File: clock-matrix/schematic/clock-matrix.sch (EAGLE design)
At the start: 85 parts, among them IC1 WS2811-SOP8, IC2 WS2811-SOP8, IC3 74HC595D, U2 ATMEGA328P-MU, X2 USB-MICROB

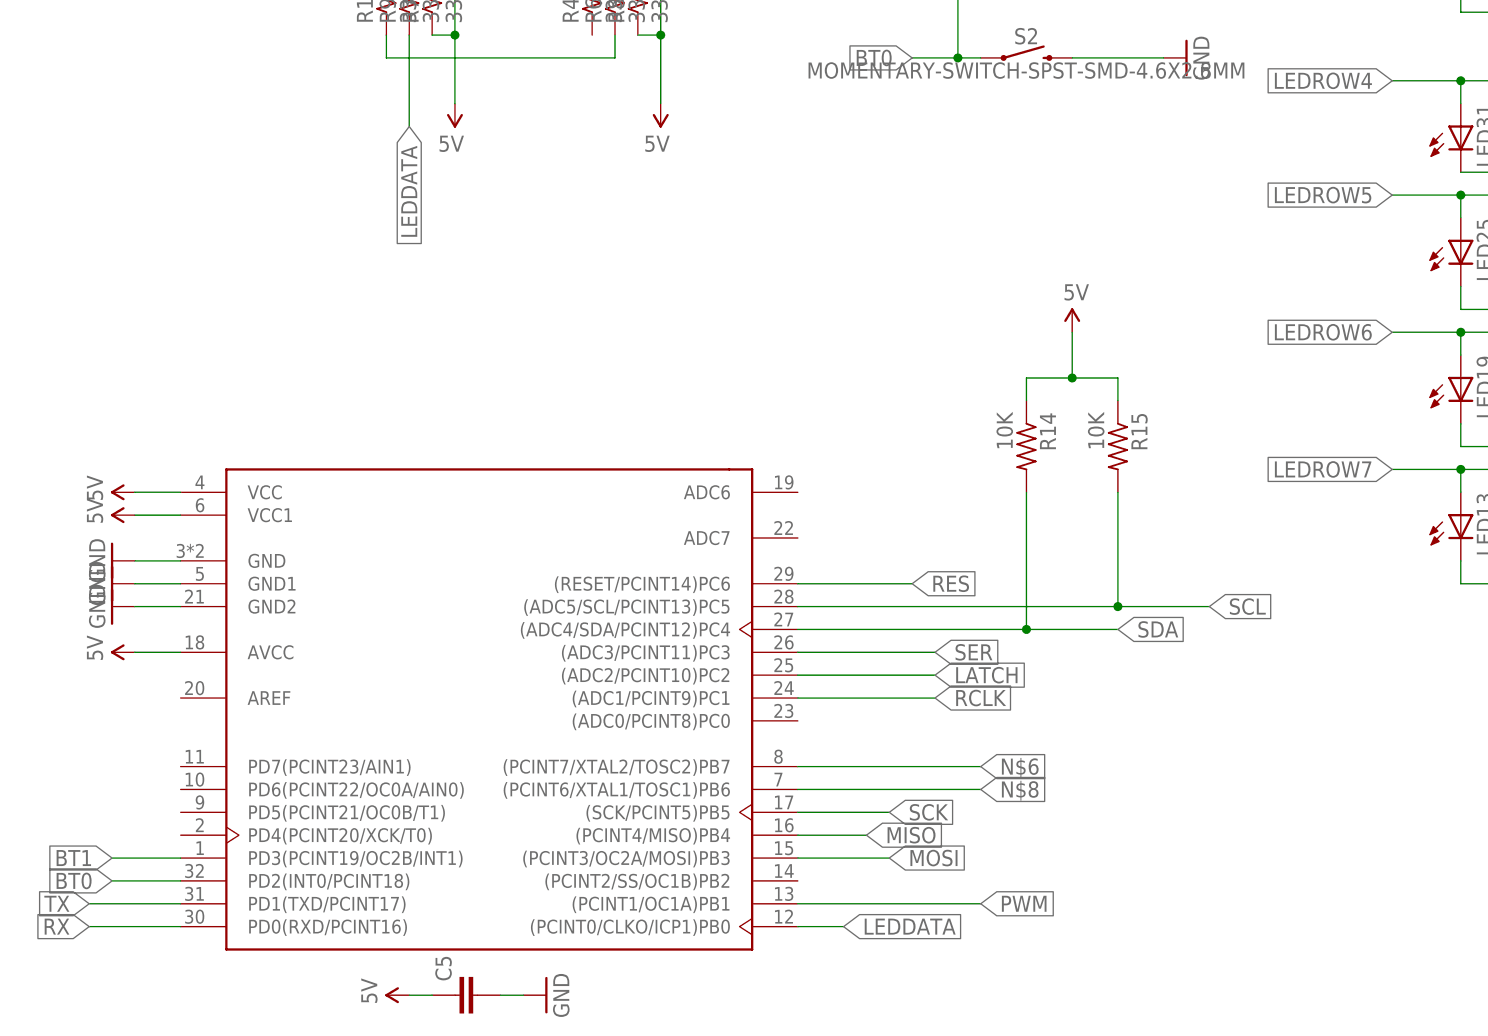
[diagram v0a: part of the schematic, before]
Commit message: Improvement, fixes and other changes
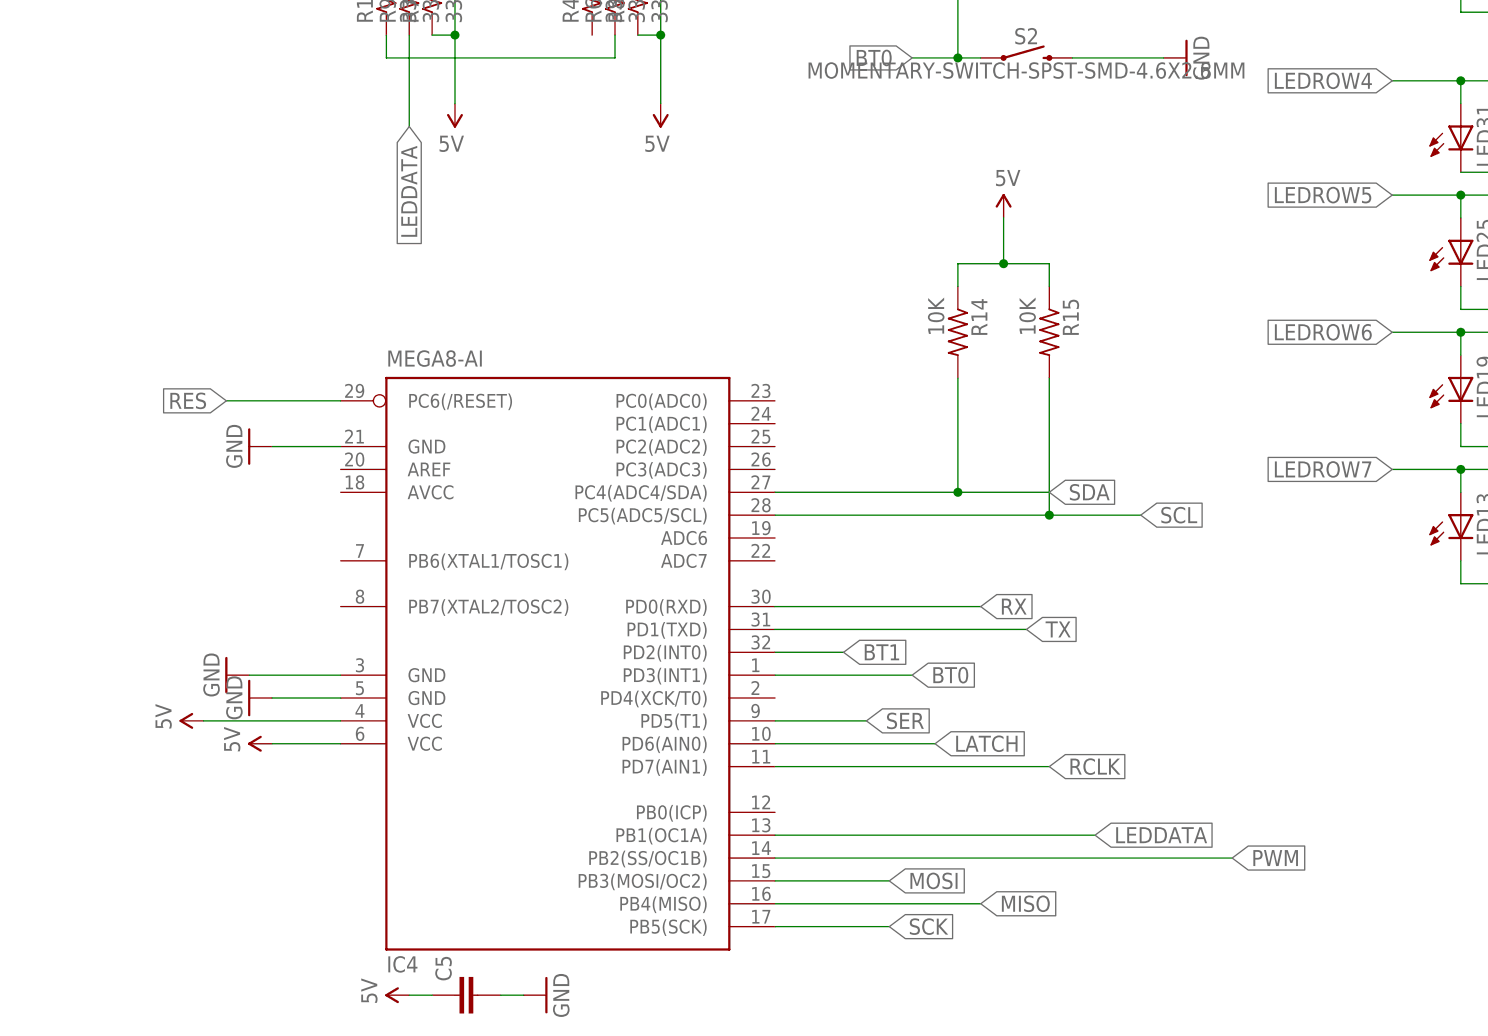
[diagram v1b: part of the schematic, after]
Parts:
- removed U2: ATMEGA328P-MU, Microcontroller:ATMEGA328P-MU
- added IC4: MEGA8-AI, atmel:MEGA8-AI
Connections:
- removed net N$6: U2.(PCINT7/XTAL2/TOSC2)PB7
- removed net N$8: U2.(PCINT6/XTAL1/TOSC1)PB6
- net 5V: now also IC4.VCC@1, IC4.VCC@2; no longer U2.AVCC, U2.VCC, U2.VCC1
- net BT0: now also IC4.PD3(INT1); no longer U2.PD2(INT0/PCINT18)
- net BT1: now also IC4.PD2(INT0); no longer U2.PD3(PCINT19/OC2B/INT1)
- net GND: now also IC4.GND, IC4.GND@1, IC4.GND@2; no longer U2.GND, U2.GND1, U2.GND2
- net LATCH: now also IC4.PD6(AIN0); no longer U2.(ADC2/PCINT10)PC2
- net LEDDATA: now also IC4.PB1(OC1A); no longer U2.(PCINT0/CLKO/ICP1)PB0
- net MISO: now also IC4.PB4(MISO); no longer U2.(PCINT4/MISO)PB4
- net MOSI: now also IC4.PB3(MOSI/OC2); no longer U2.(PCINT3/OC2A/MOSI)PB3
- net PWM: now also IC4.PB2(SS/OC1B); no longer U2.(PCINT1/OC1A)PB1
- net RCLK: now also IC4.PD7(AIN1); no longer U2.(ADC1/PCINT9)PC1
- net RES: now also IC4.PC6(/RESET); no longer U2.(RESET/PCINT14)PC6
- net RX: now also IC4.PD0(RXD); no longer U2.PD0(RXD/PCINT16)
- net SCK: now also IC4.PB5(SCK); no longer U2.(SCK/PCINT5)PB5
- net SCL: now also IC4.PC5(ADC5/SCL); no longer U2.(ADC5/SCL/PCINT13)PC5
- net SDA: now also IC4.PC4(ADC4/SDA); no longer U2.(ADC4/SDA/PCINT12)PC4
- net SER: now also IC4.PD5(T1); no longer U2.(ADC3/PCINT11)PC3
- net TX: now also IC4.PD1(TXD); no longer U2.PD1(TXD/PCINT17)
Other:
- moved on the sheet: R14, R15
